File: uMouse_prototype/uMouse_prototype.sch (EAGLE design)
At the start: 86 parts, among them IC1 LM1117IMPX-5.0, IC2 LM1117IMPX-5.0, IC3 LM1117IMPX-5.0

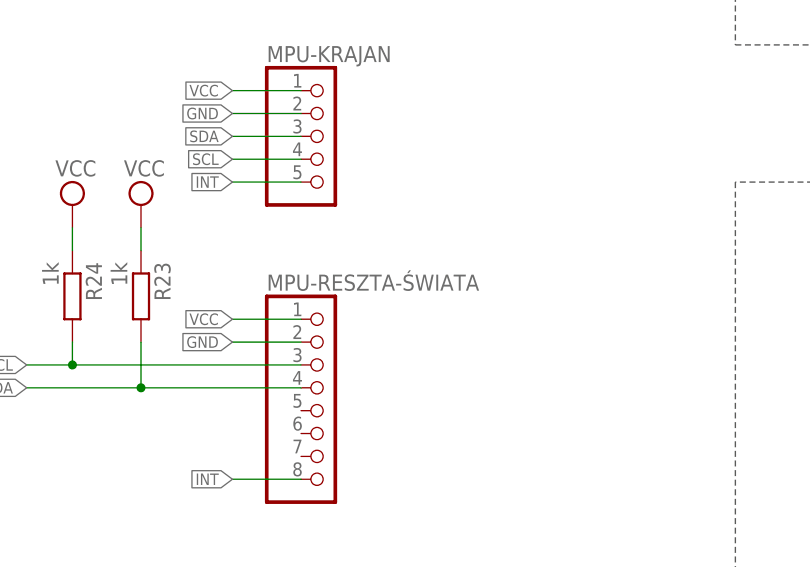
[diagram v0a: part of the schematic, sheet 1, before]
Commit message: dodane gerbery do glownej plyty prototypu
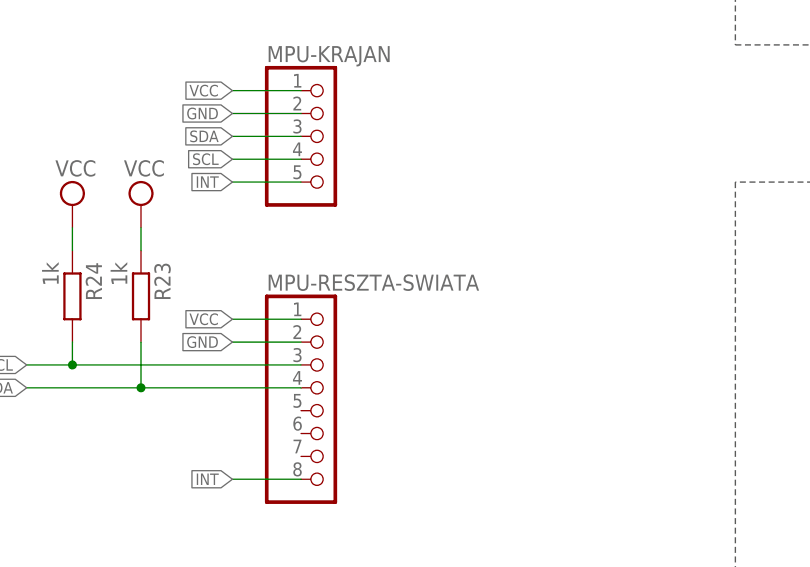
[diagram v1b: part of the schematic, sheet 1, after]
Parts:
- renumbered MPU-RESZTA-ŚWIATA to MPU-RESZTA-SWIATA
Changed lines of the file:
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@@
 <?xml version="1.0" encoding="utf-8"?>
 <!DOCTYPE eagle SYSTEM "eagle.dtd">
-<eagle version="8.5.0">
+<eagle version="8.2.0">
 <drawing>
 <settings>
 <setting alwaysvectorfont="no"/>
-<setting keepoldvectorfont="yes"/>
 <setting verticaltext="up"/>
 </settings>
@@
 <part name="U$5" library="st-morpho" deviceset="ST_MORPHO_STM32_F446RE" device=""/>
 <part name="IR1" library="adafruit" library_urn="urn:adsk.eagle:library:420" deviceset="LED" device="5MM" value="5mm IR"/>
-<part name="MPU-KRAJAN" library="pinhead" library_urn="urn:adsk.eagle:library:325" deviceset="PINHD-1X5" device="" package3d_urn="urn:adsk.eagle:package:22469/2"/>
-<part name="JP1" library="pinhead" library_urn="urn:adsk.eagle:library:325" deviceset="PINHD-2X3" device="" package3d_urn="urn:adsk.eagle:package:22462/2"/>
-<part name="JP2" library="pinhead" library_urn="urn:adsk.eagle:library:325" deviceset="PINHD-2X3" device="" package3d_urn="urn:adsk.eagle:package:22462/2"/>
+<part name="MPU-KRAJAN" library="pinhead" library_urn="urn:adsk.eagle:library:325" deviceset="PINHD-1X5" device=""/>
+<part name="JP1" library="pinhead" library_urn="urn:adsk.eagle:library:325" deviceset="PINHD-2X3" device=""/>
+<part name="JP2" library="pinhead" library_urn="urn:adsk.eagle:library:325" deviceset="PINHD-2X3" device=""/>
 <part name="GND37" library="supply1" library_urn="urn:adsk.eagle:library:371" deviceset="GND" device=""/>
 <part name="GND38" library="supply1" library_urn="urn:adsk.eagle:library:371" deviceset="GND" device=""/>
@@
 <part name="PT4" library="adafruit" library_urn="urn:adsk.eagle:library:420" deviceset="LED" device="3MM"/>
 <part name="PT5" library="adafruit" library_urn="urn:adsk.eagle:library:420" deviceset="LED" device="3MM"/>
-<part name="MPU-RESZTA-ŚWIATA" library="pinhead" library_urn="urn:adsk.eagle:library:325" deviceset="PINHD-1X8" device="" package3d_urn="urn:adsk.eagle:package:22409/2"/>
+<part name="MPU-RESZTA-SWIATA" library="pinhead" library_urn="urn:adsk.eagle:library:325" deviceset="PINHD-1X8" device=""/>
 <part name="SUPPLY29" library="supply2" library_urn="urn:adsk.eagle:library:372" deviceset="VCC" device=""/>
 <part name="SUPPLY30" library="supply2" library_urn="urn:adsk.eagle:library:372" deviceset="VCC" device=""/>
@@
 <part name="GND39" library="supply1" library_urn="urn:adsk.eagle:library:371" deviceset="GND" device=""/>
 <part name="GND40" library="supply1" library_urn="urn:adsk.eagle:library:371" deviceset="GND" device=""/>
-<part name="U$2" library="Nordic_nRF" library_urn="urn:adsk.eagle:library:169009" deviceset="INDUCTOR" device="_0805_L" package3d_urn="urn:adsk.eagle:package:169052/1"/>
+<part name="U$2" library="Nordic_nRF" library_urn="urn:adsk.eagle:library:169009" deviceset="INDUCTOR" device="_0805_L"/>
 <part name="SUPPLY31" library="supply2" library_urn="urn:adsk.eagle:library:372" deviceset="VCC" device=""/>
 <part name="C27" library="rcl" library_urn="urn:adsk.eagle:library:334" deviceset="C-EU" device="C0805K" value="100nF 6.3V"/>
 <part name="GND41" library="supply1" library_urn="urn:adsk.eagle:library:371" deviceset="GND" device=""/>
 <part name="GND42" library="supply1" library_urn="urn:adsk.eagle:library:371" deviceset="GND" device=""/>
-<part name="JP3" library="pinhead" library_urn="urn:adsk.eagle:library:325" deviceset="PINHD-1X2" device="" package3d_urn="urn:adsk.eagle:package:22435/2"/>
-<part name="JP4" library="pinhead" library_urn="urn:adsk.eagle:library:325" deviceset="PINHD-1X2" device="" package3d_urn="urn:adsk.eagle:package:22435/2"/>
+<part name="JP3" library="pinhead" library_urn="urn:adsk.eagle:library:325" deviceset="PINHD-1X2" device=""/>
+<part name="JP4" library="pinhead" library_urn="urn:adsk.eagle:library:325" deviceset="PINHD-1X2" device=""/>
 <part name="IC3" library="lm1117" deviceset="LM1117IMPX-*" device="" technology="5.0"/>
 <part name="C28" library="rcl" library_urn="urn:adsk.eagle:library:334" deviceset="C-EU" device="C0805K" value="1uF 16V"/>
@@
 <part name="C30" library="rcl" library_urn="urn:adsk.eagle:library:334" deviceset="C-EU" device="C0805K" value="100nF 6.3V"/>
 <part name="GND46" library="supply1" library_urn="urn:adsk.eagle:library:371" deviceset="GND" device=""/>
-<part name="JP5" library="pinhead" library_urn="urn:adsk.eagle:library:325" deviceset="PINHD-1X6" device="" package3d_urn="urn:adsk.eagle:package:22472/2"/>
+<part name="JP5" library="pinhead" library_urn="urn:adsk.eagle:library:325" deviceset="PINHD-1X6" device=""/>
 <part name="R25" library="rcl" library_urn="urn:adsk.eagle:library:334" deviceset="R-EU_" device="M0805" value="0R"/>
 <part name="R23" library="rcl" library_urn="urn:adsk.eagle:library:334" deviceset="R-EU_" device="M0805" value="1k"/>
@@
 <instance part="PT4" gate="G$1" x="541.02" y="15.24"/>
 <instance part="PT5" gate="G$1" x="614.68" y="15.24"/>
-<instance part="MPU-RESZTA-ŚWIATA" gate="A" x="226.06" y="40.64"/>
+<instance part="MPU-RESZTA-SWIATA" gate="A" x="226.06" y="40.64"/>
 <instance part="SUPPLY29" gate="G$1" x="-12.7" y="149.86"/>
 <instance part="SUPPLY30" gate="G$1" x="-12.7" y="111.76" rot="MR0"/>
@@
 <wire x1="223.52" y1="48.26" x2="215.9" y2="48.26" width="0.1524" layer="91"/>
 <label x="215.9" y="48.26" size="1.27" layer="95" rot="R180" xref="yes"/>
-<pinref part="MPU-RESZTA-ŚWIATA" gate="A" pin="2"/>
+<pinref part="MPU-RESZTA-SWIATA" gate="A" pin="2"/>
 </segment>
 <segment>
@@
 <wire x1="223.52" y1="50.8" x2="215.9" y2="50.8" width="0.1524" layer="91"/>
 <label x="215.9" y="50.8" size="1.27" layer="95" rot="R180" xref="yes"/>
-<pinref part="MPU-RESZTA-ŚWIATA" gate="A" pin="1"/>
+<pinref part="MPU-RESZTA-SWIATA" gate="A" pin="1"/>
 </segment>
 <segment>
@@
 <wire x1="223.52" y1="45.72" x2="198.12" y2="45.72" width="0.1524" layer="91"/>
 <label x="193.04" y="45.72" size="1.27" layer="95" rot="R180" xref="yes"/>
-<pinref part="MPU-RESZTA-ŚWIATA" gate="A" pin="3"/>
+<pinref part="MPU-RESZTA-SWIATA" gate="A" pin="3"/>
 <pinref part="R24" gate="G$1" pin="2"/>
 <wire x1="198.12" y1="45.72" x2="193.04" y2="45.72" width="0.1524" layer="91"/>
@@
 <wire x1="223.52" y1="43.18" x2="205.74" y2="43.18" width="0.1524" layer="91"/>
 <label x="193.04" y="43.18" size="1.27" layer="95" rot="R180" xref="yes"/>
-<pinref part="MPU-RESZTA-ŚWIATA" gate="A" pin="4"/>
+<pinref part="MPU-RESZTA-SWIATA" gate="A" pin="4"/>
 <pinref part="R23" gate="G$1" pin="2"/>
 <wire x1="205.74" y1="43.18" x2="193.04" y2="43.18" width="0.1524" layer="91"/>
@@
 <segment>
 <label x="215.9" y="33.02" size="1.27" layer="95" rot="R180" xref="yes"/>
-<pinref part="MPU-RESZTA-ŚWIATA" gate="A" pin="8"/>
+<pinref part="MPU-RESZTA-SWIATA" gate="A" pin="8"/>
 <wire x1="223.52" y1="33.02" x2="215.9" y2="33.02" width="0.1524" layer="91"/>
 </segment>
@@
 </note>
 <note version="8.2" severity="warning">
-Since Version 8.2, EAGLE supports online libraries. The ids
+Since Version 8.2, Eagle supports online libraries. The ids
 of those online libraries will not be understood (or retained)
 with this version.
 </note>
-<note version="8.3" severity="warning">
-Since Version 8.3, EAGLE supports URNs for individual library
-assets (packages, symbols, and devices). The URNs of those assets
-will not be understood (or retained) with this version.
-</note>
-<note version="8.3" severity="warning">
-Since Version 8.3, EAGLE supports the association of 3D packages
-with devices in libraries, schematics, and board files. Those 3D
-packages will not be understood (or retained) with this version.
-</note>
 </compatibility>
